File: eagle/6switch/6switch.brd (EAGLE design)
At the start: 57.1 x 71.4 mm, 13 parts, among them IC1 MCP23017SP, J1 RELAYBRD, Q1 BC548, X1 Sw1, X2 Sw7, X3 Sw5, X4 Sw4, X5 Sw3, X6 Sw2

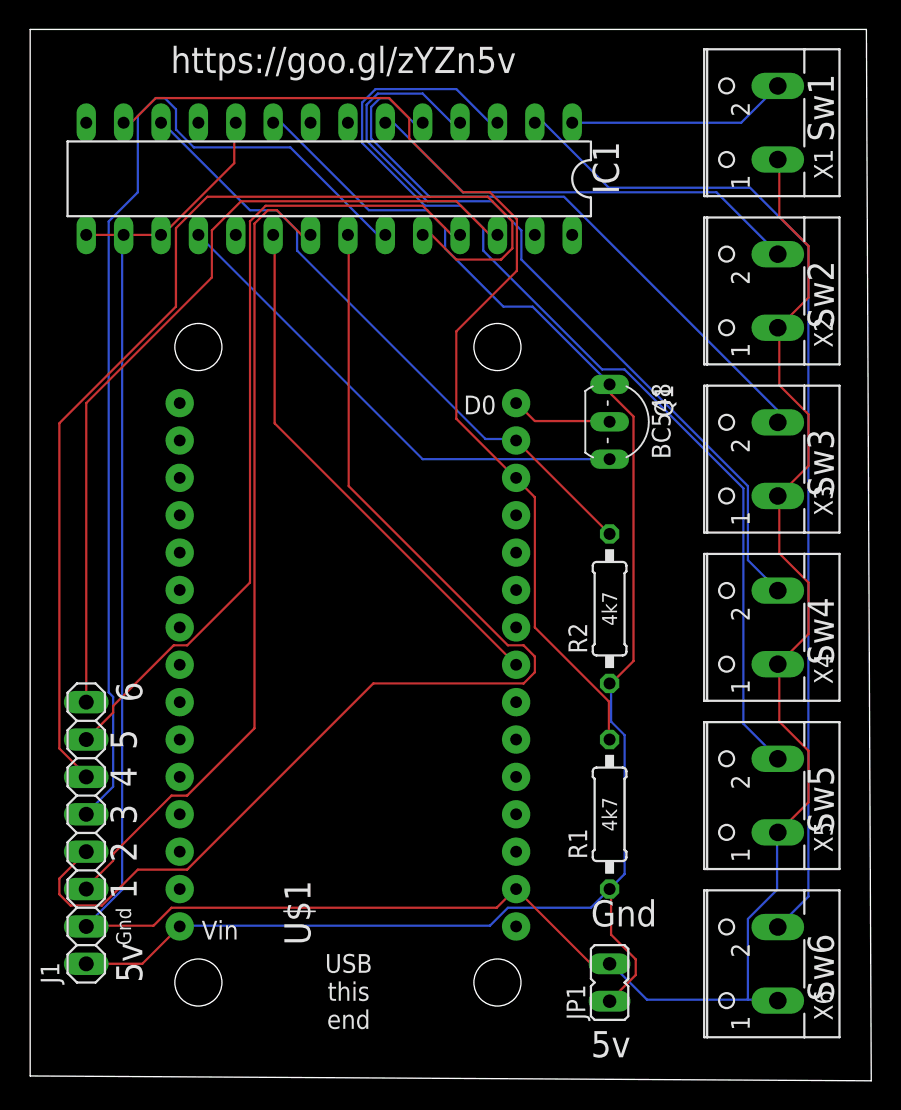
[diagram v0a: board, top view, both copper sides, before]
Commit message: dru changed
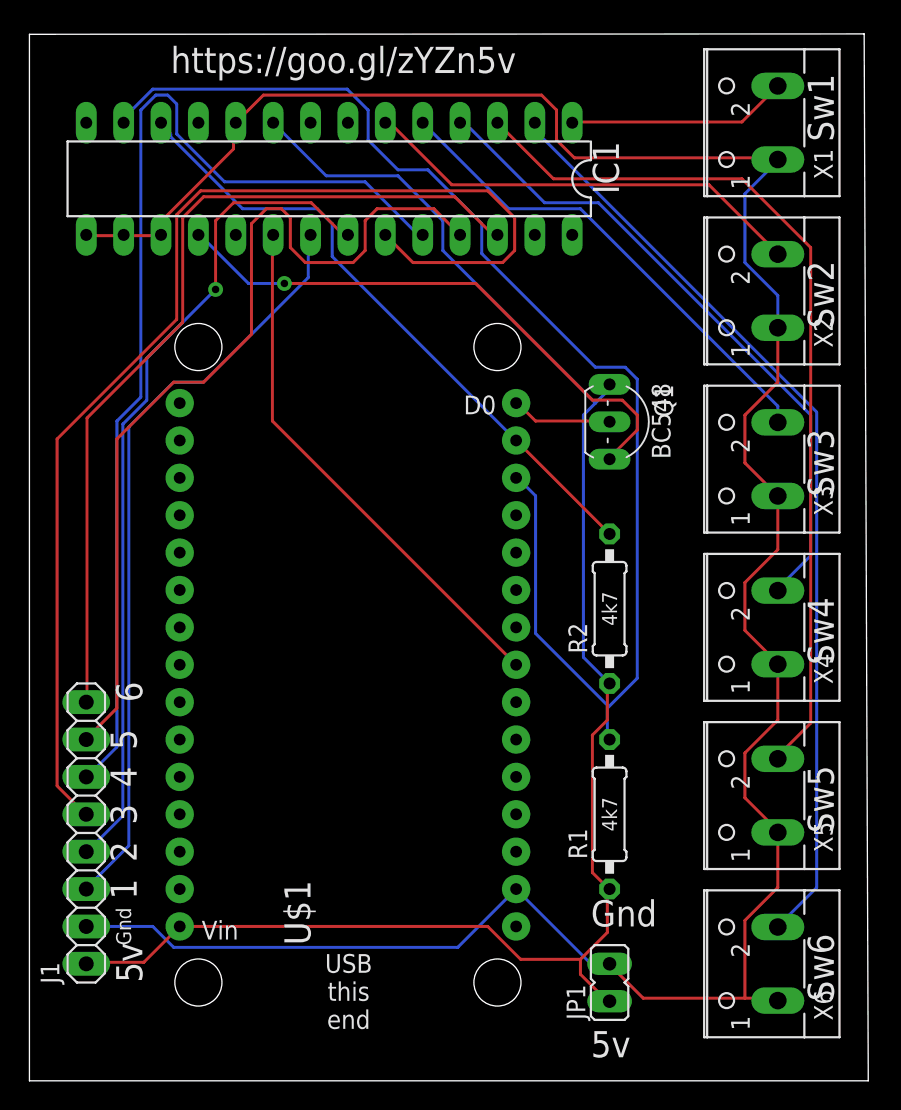
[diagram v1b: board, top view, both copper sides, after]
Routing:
- net N$11: track 78.5 -> 57.0 mm, vias 0 -> 1
- net N$4: track 73.0 -> 90.3 mm
- net N$12: track 71.1 -> 81.5 mm
- net N$9: track 54.6 -> 45.0 mm
- net N$16: track 42.7 -> 33.2 mm
- net N$8: track 69.1 -> 60.5 mm
- net GND: track 179.1 -> 173.3 mm
- net N$14: track 55.9 -> 61.6 mm
- net N$6: track 69.2 -> 63.7 mm
- net N$2: track 34.3 -> 38.6 mm, vias 0 -> 1
- net N$10: track 55.5 -> 52.0 mm
- net N$13: track 74.7 -> 71.6 mm
- net N$15: track 56.8 -> 58.8 mm
- net VCC: track 114.4 -> 112.8 mm
- net N$3: track 42.9 -> 43.5 mm
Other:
- board size 57.1 x 71.4 mm -> 57 x 71.1 mm
